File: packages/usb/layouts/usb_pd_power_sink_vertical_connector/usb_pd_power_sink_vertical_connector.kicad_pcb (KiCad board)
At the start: 2 copper layers, 8 parts, among them U2 2.9V

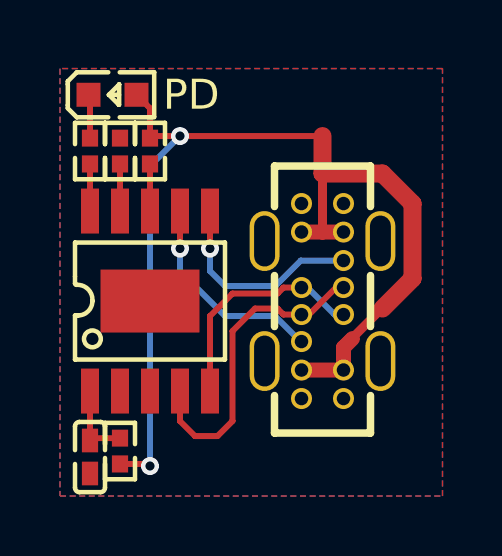
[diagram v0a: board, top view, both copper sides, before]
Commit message: WIP update usb
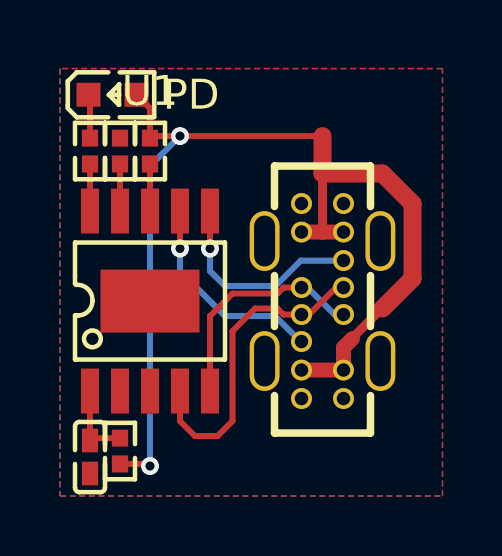
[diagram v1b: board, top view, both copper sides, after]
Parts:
- C1: value 1µF ±10% 16V X5R -> 1µF ±10% 25V X5R; footprint atopile:C0402-b3ef17 -> Samsung_Electro_Mechanics_CL05A105KA5NQNC:C0402
- R1, R2, R4: footprint atopile:R0402-56259e -> UNI_ROYAL_0402WGF1002TCE:R0402
- R3: footprint atopile:R0402-56259e -> UNI_ROYAL_0402WGF1001TCE:R0402
- U1: footprint atopile:ESSOP-10_L4.9-W3.9-P1.0-LS6.0-TL-EP-20a8ca -> WCH_CH224K:ESSOP-10_L4.9-W3.9-P1.0-LS6.0-TL-EP
- U2: footprint lib:LED0603-RD -> Hubei_KENTO_Elec_Blue_light_0603:LED0603-RD
- X1: footprint atopile:USB-C-TH_TYPE-C-USB-14P-1a34cb -> Jing_Extension_of_the_Electronic_Co_918_418K2022Y40000:USB-C-TH_TYPE-C-USB-14P
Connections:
- R2 pad 2: pd_trigger-line-1 -> pd_trigger-line
- R4 pad 1: pd_trigger-line -> pd_trigger-line-1
- U1 pad 2: pd_trigger.controller-line -> pd_trigger.controller-line-1
- U1 pad 3: pd_trigger.controller-line-1 -> pd_trigger.controller-line
- U1 pad 4: line -> line-1
- U1 pad 5: line-3 -> line
- U1 pad 6: line-1 -> line-2
- U1 pad 7: line-2 -> line-3
- U1 pad 8: pd_trigger-line-1 -> pd_trigger-line
- U1 pad 9: pd_trigger-line -> pd_trigger-line-1
- X1 pad 10: line-3 -> line
- X1 pad 11: line -> line-1
- X1 pad 12: line-2 -> line-3
- X1 pad 3: line-3 -> line
- X1 pad 4: line -> line-1
- X1 pad 5: line-1 -> line-2
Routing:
- net line-1: track 7.01 -> 10.6 mm, vias 1 -> 0
- net line: track 10.6 -> 7.72 mm
- net line-3: track 7.72 -> 7.02 mm, vias 0 -> 1
